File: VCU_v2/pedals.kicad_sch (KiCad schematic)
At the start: 21 parts, among them U10 TSB712AIDT, U9 TSB712AIDT

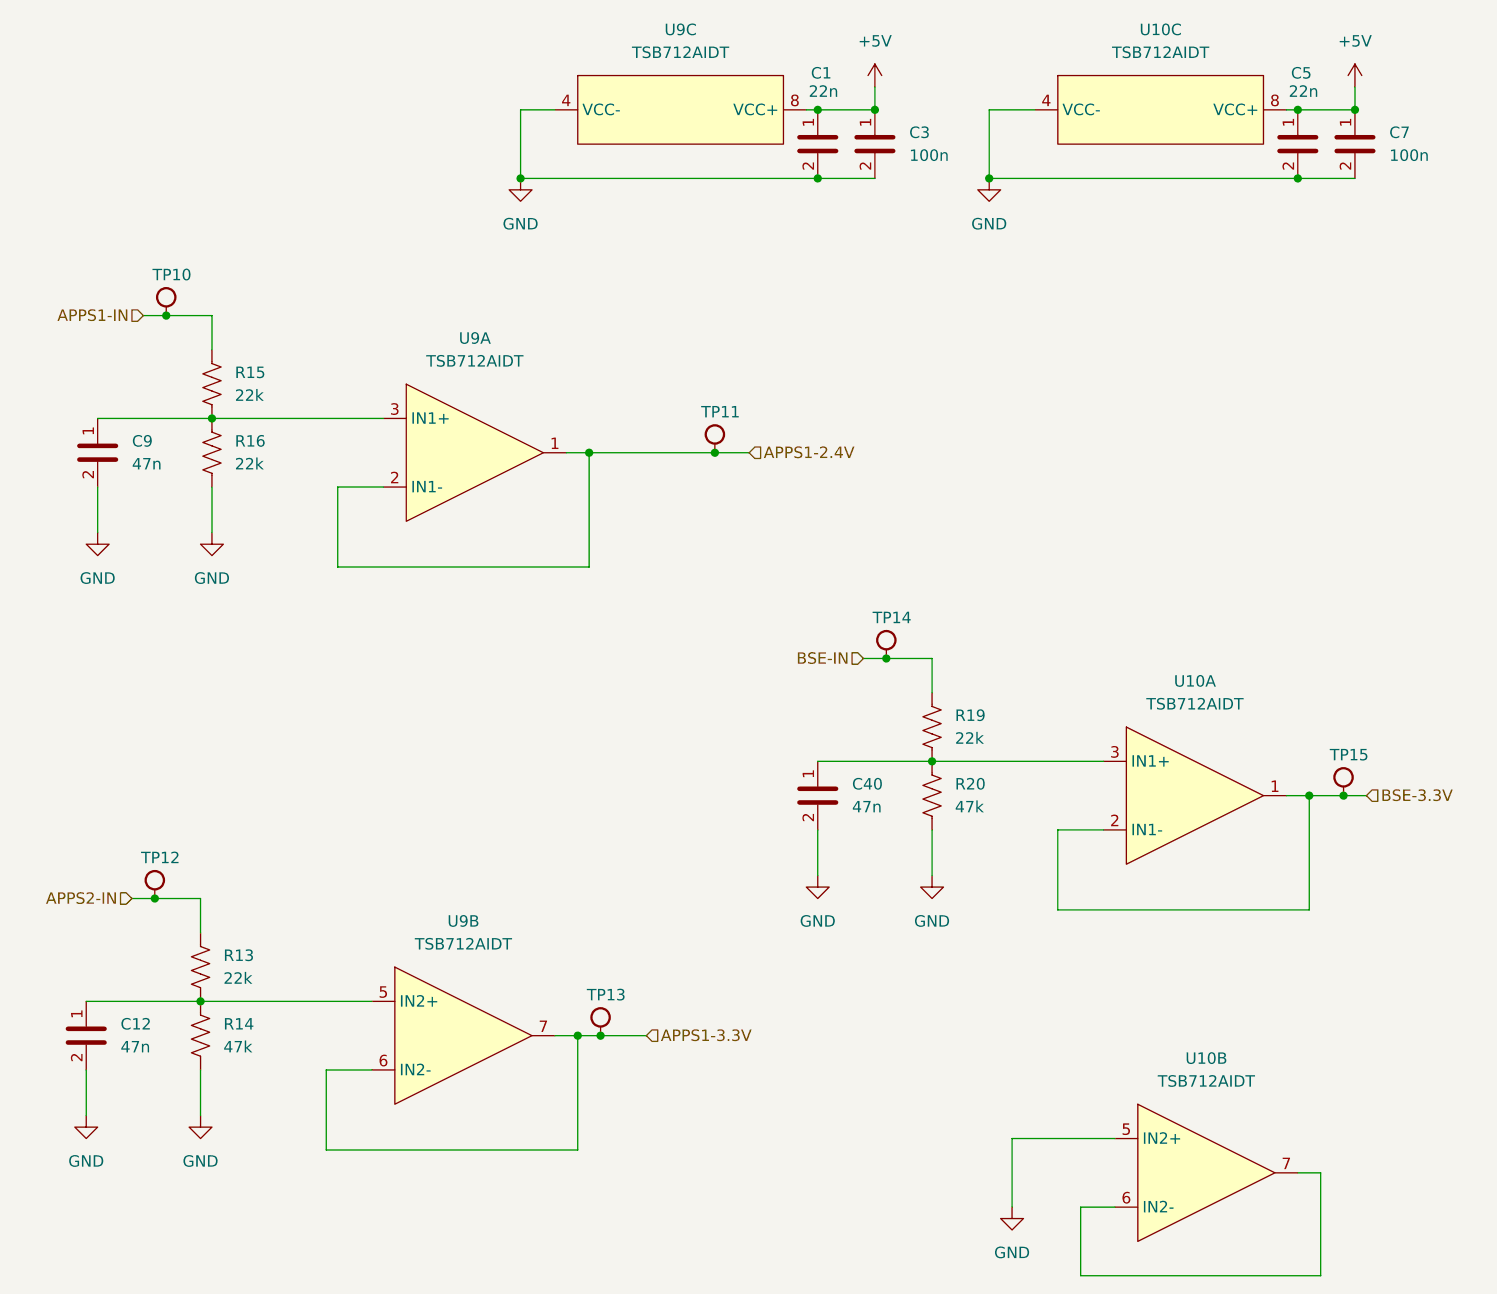
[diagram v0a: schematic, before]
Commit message: vcu v2 schematics done
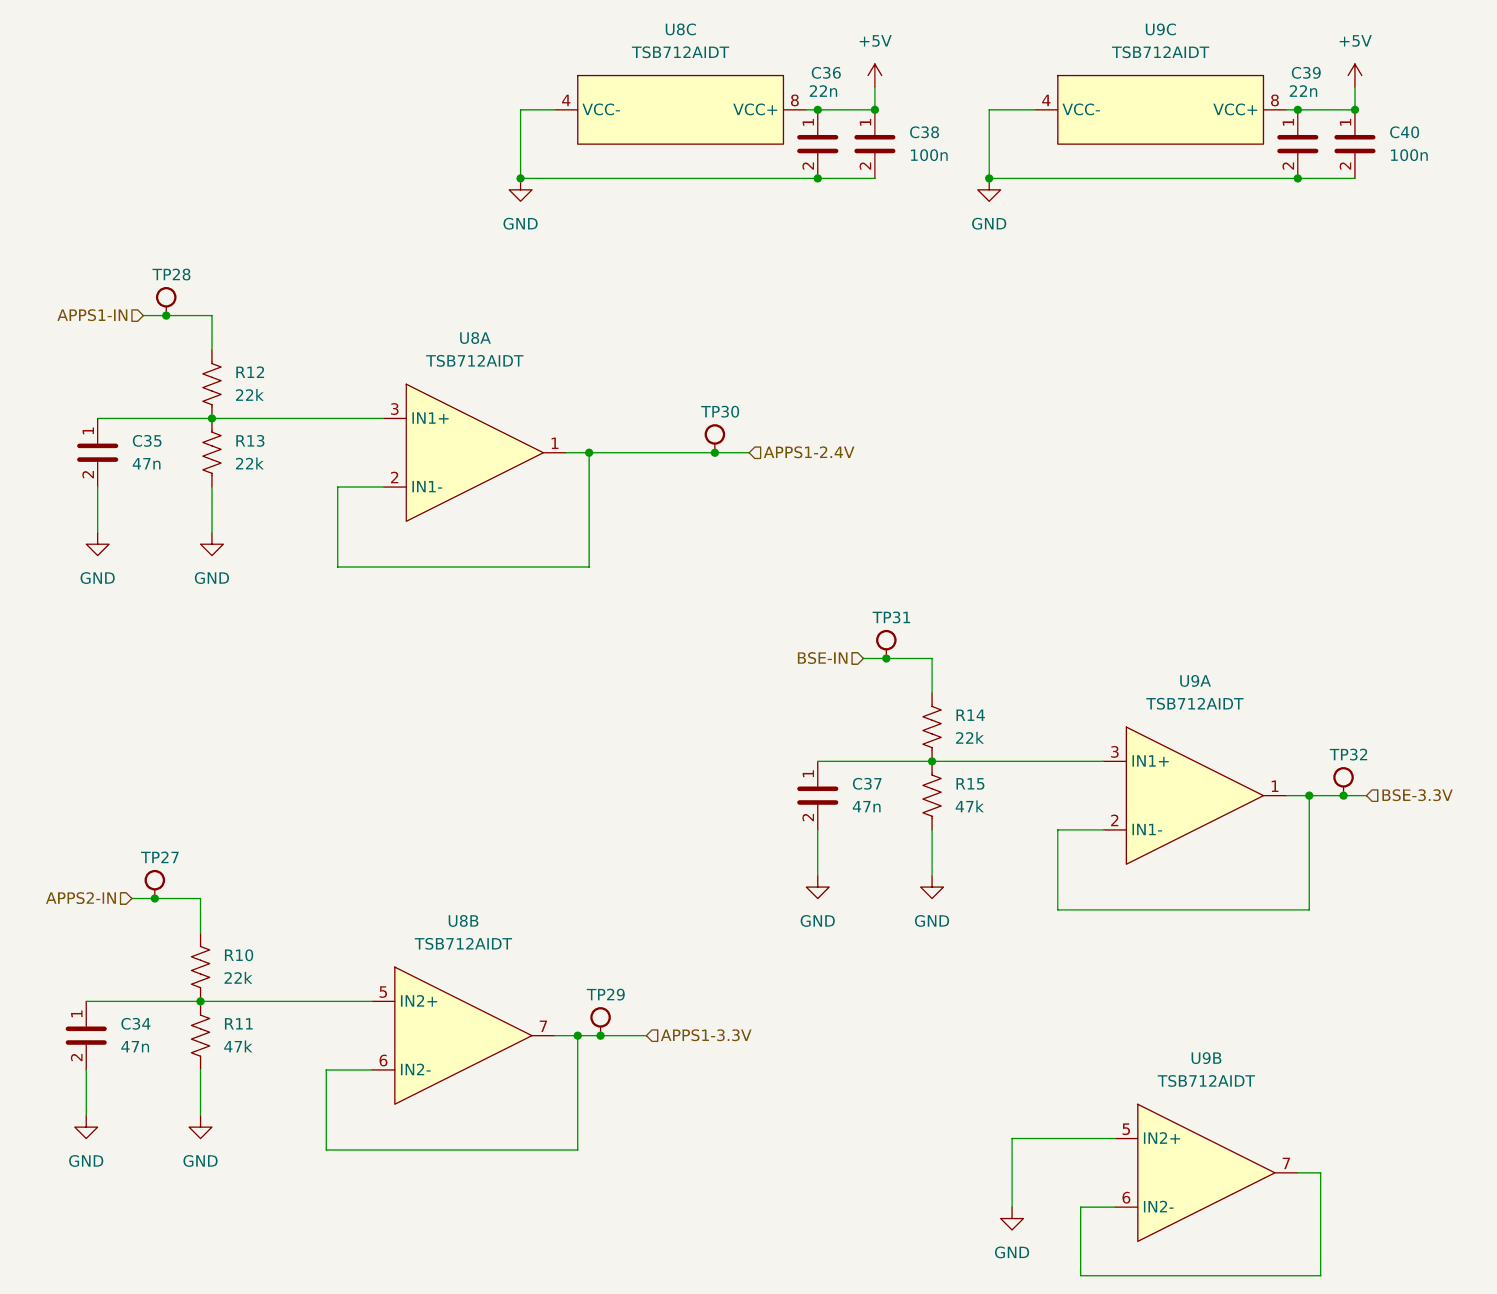
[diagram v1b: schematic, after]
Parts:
- renumbered C12 to C34, C9 to C35, C1 to C36, C40 to C37, C3 to C38, C5 to C39, C7 to C40, R13 to R10, R14 to R11, R15 to R12, R16 to R13, R19 to R14, R20 to R15, TP12 to TP27, TP10 to TP28, TP13 to TP29, TP11 to TP30, TP14 to TP31, TP15 to TP32, U9 to U8, U10 to U9

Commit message: placements friggin 80% friggin done shoutout epstein
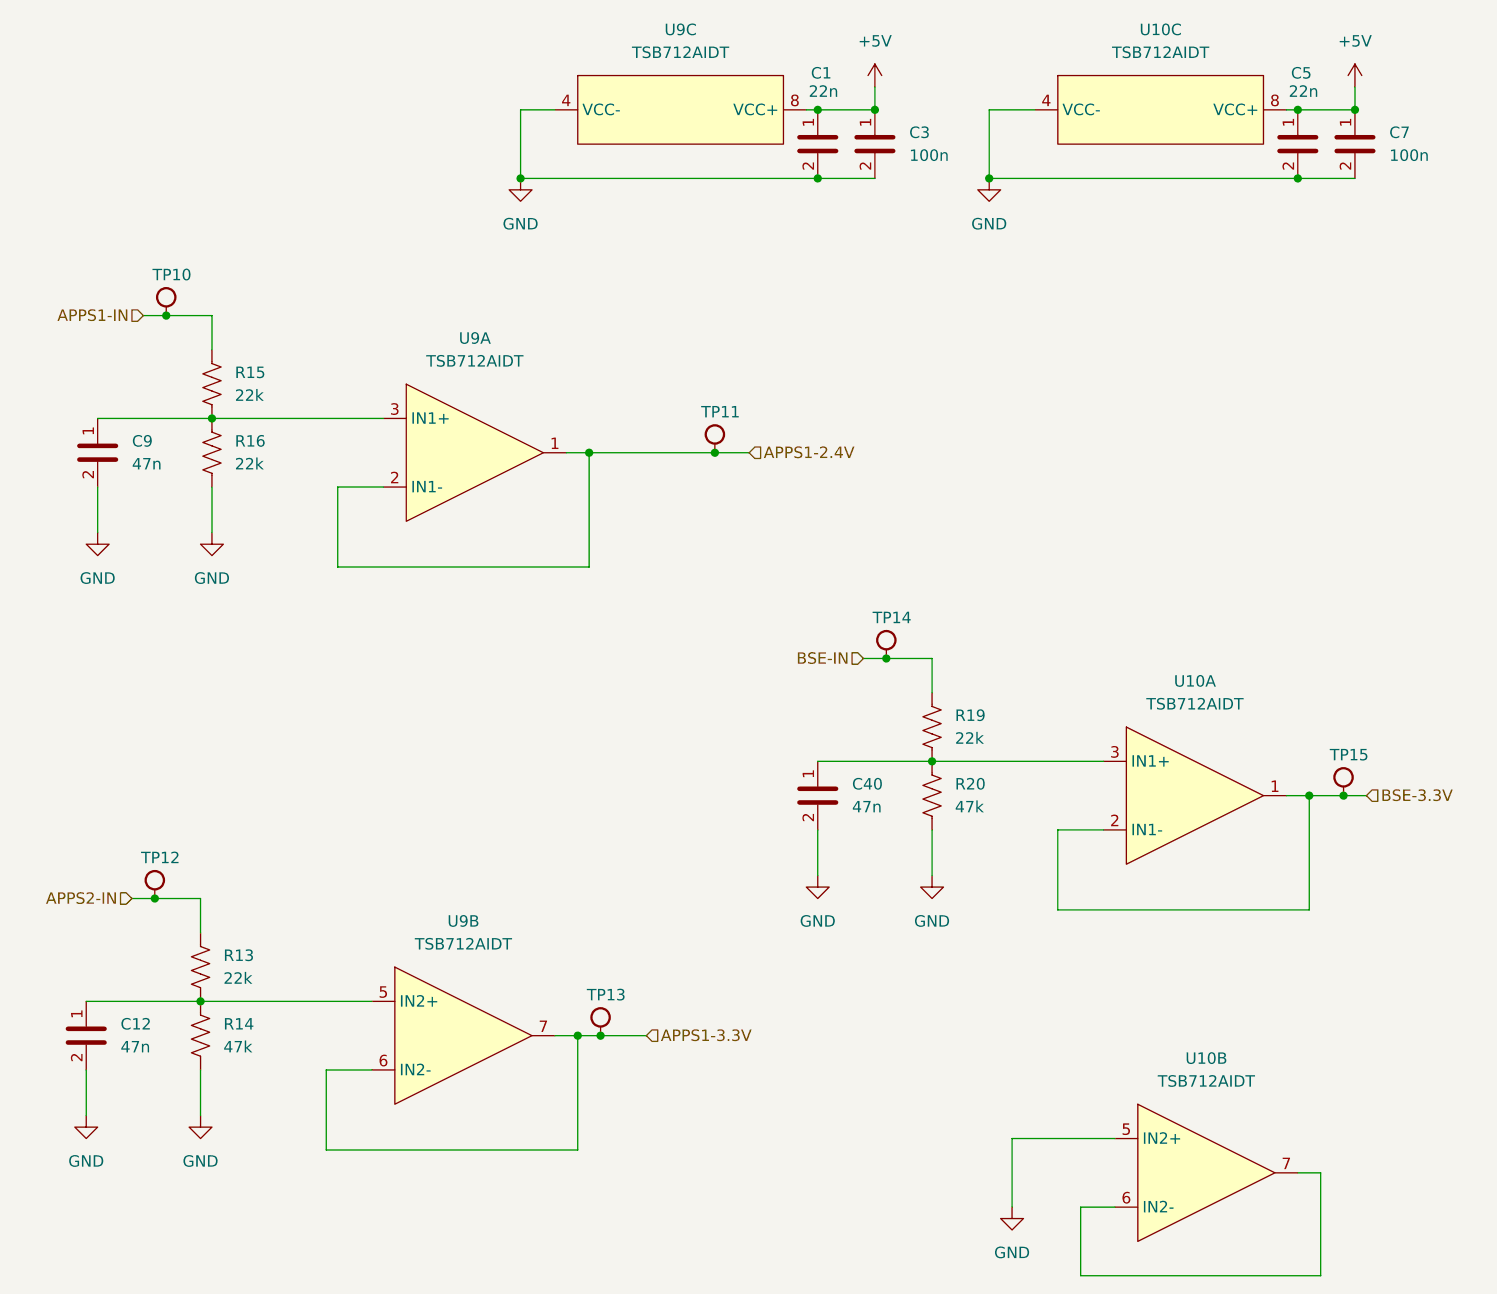
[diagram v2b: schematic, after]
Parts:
- renumbered C36 to C1, C34 to C12, C38 to C3, C37 to C40, C39 to C5, C40 to C7, C35 to C9, R10 to R13, R11 to R14, R12 to R15, R13 to R16, R14 to R19, R15 to R20, TP28 to TP10, TP30 to TP11, TP27 to TP12, TP29 to TP13, TP31 to TP14, TP32 to TP15, U9 to U10, U8 to U9
